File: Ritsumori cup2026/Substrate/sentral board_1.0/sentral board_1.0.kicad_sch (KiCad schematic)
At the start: 9 parts, among them J1 Conn_02x10_Odd_Even, J2 Conn_02x05_Counter_Clockwise, J3 Conn_01x04_Socket, J4 Conn_01x05_Socket, J5 Conn_01x02_Socket, J6 Conn_01x02_Socket, J7 Conn_01x02_Socket, J8 Conn_01x02_Socket, J9 Conn_01x04_Socket

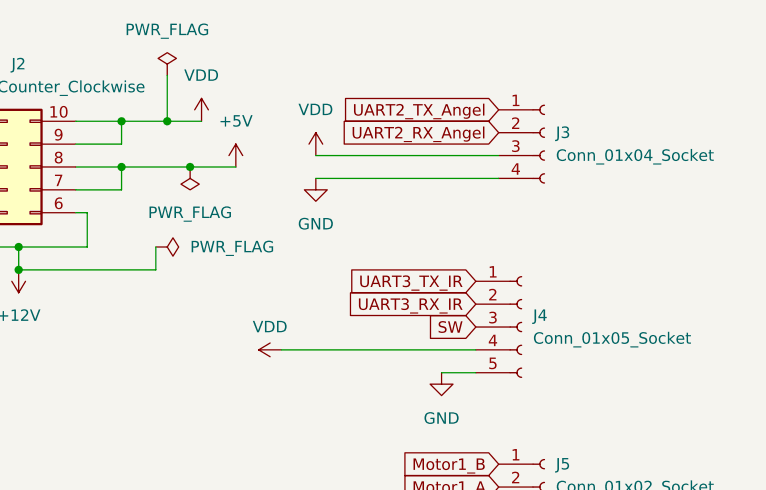
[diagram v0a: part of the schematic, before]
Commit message: Auto Backup: 2026/03/09 13:07:55.49
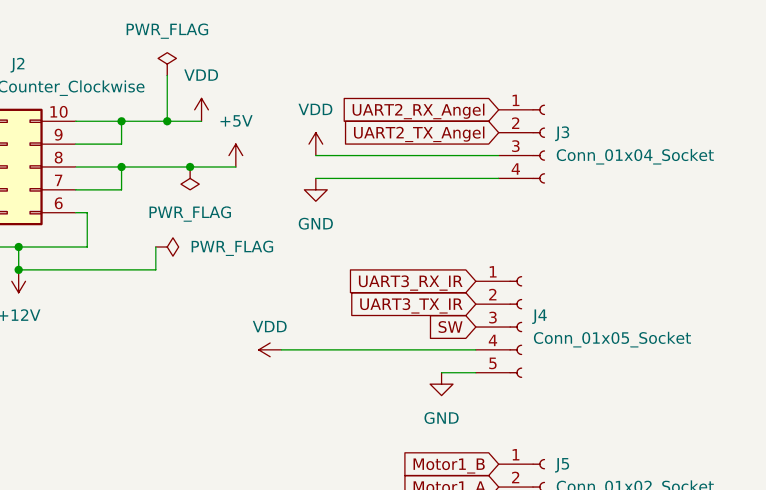
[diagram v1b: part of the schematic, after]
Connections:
- net UART2_RX_Angel: now also J3.1 (Pin_1); no longer J3.2 (Pin_2)
- net UART2_TX_Angel: now also J3.2 (Pin_2); no longer J3.1 (Pin_1)
- net UART3_RX_IR: now also J4.1 (Pin_1); no longer J4.2 (Pin_2)
- net UART3_TX_IR: now also J4.2 (Pin_2); no longer J4.1 (Pin_1)
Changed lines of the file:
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@@
 	(global_label "UART2_RX_Angel"
 		(shape input)
+		(at 228.6 46.99 180)
+		(fields_autoplaced yes)
+		(effects
+			(font
+				(size 1.27 1.27)
+			)
+			(justify right)
+		)
+		(property "Intersheetrefs" "${INTERSHEET_REFS}"
+			(at 210.1935 46.99 0)
+			(effects
+				(font
+					(size 1.27 1.27)
+				)
+				(justify right)
+				(hide yes)
+			)
+		)
+	)
+	(global_label "Motor4_B"
+		(shape input)
+		(at 161.29 85.09 0)
+		(fields_autoplaced yes)
+		(effects
+			(font
+				(size 1.27 1.27)
+			)
+			(justify left)
+		)
+		(property "Intersheetrefs" "${INTERSHEET_REFS}"
+			(at 172.9836 85.09 0)
+			(effects
+				(font
+					(size 1.27 1.27)
+				)
+				(justify left)
+				(hide yes)
+			)
+		)
+	)
+	(global_label "Motor2_B"
+		(shape input)
+		(at 228.6 91.44 180)
+		(fields_autoplaced yes)
+		(effects
+			(font
+				(size 1.27 1.27)
+			)
+			(justify right)
+		)
+		(property "Intersheetrefs" "${INTERSHEET_REFS}"
+			(at 216.9064 91.44 0)
+			(effects
+				(font
+					(size 1.27 1.27)
+				)
+				(justify right)
+				(hide yes)
+			)
+		)
+	)
+	(global_label "UART3_TX_IR"
+		(shape input)
+		(at 226.06 68.58 180)
+		(fields_autoplaced yes)
+		(effects
+			(font
+				(size 1.27 1.27)
+			)
+			(justify right)
+		)
+		(property "Intersheetrefs" "${INTERSHEET_REFS}"
+			(at 211.2215 68.58 0)
+			(effects
+				(font
+					(size 1.27 1.27)
+				)
+				(justify right)
+				(hide yes)
+			)
+		)
+	)
+	(global_label "UART3_RX_IR"
+		(shape input)
+		(at 226.06 66.04 180)
+		(fields_autoplaced yes)
+		(effects
+			(font
+				(size 1.27 1.27)
+			)
+			(justify right)
+		)
+		(property "Intersheetrefs" "${INTERSHEET_REFS}"
+			(at 210.9191 66.04 0)
+			(effects
+				(font
+					(size 1.27 1.27)
+				)
+				(justify right)
+				(hide yes)
+			)
+		)
+	)
+	(global_label "Motor1_B"
+		(shape input)
+		(at 228.6 86.36 180)
+		(fields_autoplaced yes)
+		(effects
+			(font
+				(size 1.27 1.27)
+			)
+			(justify right)
+		)
+		(property "Intersheetrefs" "${INTERSHEET_REFS}"
+			(at 216.9064 86.36 0)
+			(effects
+				(font
+					(size 1.27 1.27)
+				)
+				(justify right)
+				(hide yes)
+			)
+		)
+	)
+	(global_label "SW"
+		(shape input)
+		(at 161.29 82.55 0)
+		(fields_autoplaced yes)
+		(effects
+			(font
+				(size 1.27 1.27)
+			)
+			(justify left)
+		)
+		(property "Intersheetrefs" "${INTERSHEET_REFS}"
+			(at 166.9361 82.55 0)
+			(effects
+				(font
+					(size 1.27 1.27)
+				)
+				(justify left)
+				(hide yes)
+			)
+		)
+	)
+	(global_label "Motor2_A"
+		(shape input)
+		(at 228.6 93.98 180)
+		(fields_autoplaced yes)
+		(effects
+			(font
+				(size 1.27 1.27)
+			)
+			(justify right)
+		)
+		(property "Intersheetrefs" "${INTERSHEET_REFS}"
+			(at 217.0878 93.98 0)
+			(effects
+				(font
+					(size 1.27 1.27)
+				)
+				(justify right)
+				(hide yes)
+			)
+		)
+	)
+	(global_label "Motor1_A"
+		(shape input)
+		(at 161.29 102.87 0)
+		(fields_autoplaced yes)
+		(effects
+			(font
+				(size 1.27 1.27)
+			)
+			(justify left)
+		)
+		(property "Intersheetrefs" "${INTERSHEET_REFS}"
+			(at 172.8022 102.87 0)
+			(effects
+				(font
+					(size 1.27 1.27)
+				)
+				(justify left)
+				(hide yes)
+			)
+		)
+	)
+	(global_label "Motor3_B"
+		(shape input)
+		(at 228.6 96.52 180)
+		(fields_autoplaced yes)
+		(effects
+			(font
+				(size 1.27 1.27)
+			)
+			(justify right)
+		)
+		(property "Intersheetrefs" "${INTERSHEET_REFS}"
+			(at 216.9064 96.52 0)
+			(effects
+				(font
+					(size 1.27 1.27)
+				)
+				(justify right)
+				(hide yes)
+			)
+		)
+	)
+	(global_label "UART2_TX_Angel"
+		(shape input)
 		(at 228.6 49.53 180)
 		(fields_autoplaced yes)
@@
 		)
 		(property "Intersheetrefs" "${INTERSHEET_REFS}"
-			(at 210.1935 49.53 0)
-			(effects
-				(font
-					(size 1.27 1.27)
-				)
-				(justify right)
-				(hide yes)
-			)
-		)
-	)
-	(global_label "Motor4_B"
-		(shape input)
-		(at 161.29 85.09 0)
-		(fields_autoplaced yes)
-		(effects
-			(font
-				(size 1.27 1.27)
-			)
-			(justify left)
-		)
-		(property "Intersheetrefs" "${INTERSHEET_REFS}"
-			(at 172.9836 85.09 0)
-			(effects
-				(font
-					(size 1.27 1.27)
-				)
-				(justify left)
-				(hide yes)
-			)
-		)
-	)
-	(global_label "Motor2_B"
-		(shape input)
-		(at 228.6 91.44 180)
-		(fields_autoplaced yes)
-		(effects
-			(font
-				(size 1.27 1.27)
-			)
-			(justify right)
-		)
-		(property "Intersheetrefs" "${INTERSHEET_REFS}"
-			(at 216.9064 91.44 0)
-			(effects
-				(font
-					(size 1.27 1.27)
-				)
-				(justify right)
-				(hide yes)
-			)
-		)
-	)
-	(global_label "UART3_TX_IR"
-		(shape input)
-		(at 226.06 66.04 180)
-		(fields_autoplaced yes)
-		(effects
-			(font
-				(size 1.27 1.27)
-			)
-			(justify right)
-		)
-		(property "Intersheetrefs" "${INTERSHEET_REFS}"
-			(at 211.2215 66.04 0)
-			(effects
-				(font
-					(size 1.27 1.27)
-				)
-				(justify right)
-				(hide yes)
-			)
-		)
-	)
-	(global_label "UART3_RX_IR"
-		(shape input)
-		(at 226.06 68.58 180)
-		(fields_autoplaced yes)
-		(effects
-			(font
-				(size 1.27 1.27)
-			)
-			(justify right)
-		)
-		(property "Intersheetrefs" "${INTERSHEET_REFS}"
-			(at 210.9191 68.58 0)
-			(effects
-				(font
-					(size 1.27 1.27)
-				)
-				(justify right)
-				(hide yes)
-			)
-		)
-	)
-	(global_label "Motor1_B"
-		(shape input)
-		(at 228.6 86.36 180)
-		(fields_autoplaced yes)
-		(effects
-			(font
-				(size 1.27 1.27)
-			)
-			(justify right)
-		)
-		(property "Intersheetrefs" "${INTERSHEET_REFS}"
-			(at 216.9064 86.36 0)
-			(effects
-				(font
-					(size 1.27 1.27)
-				)
-				(justify right)
-				(hide yes)
-			)
-		)
-	)
-	(global_label "SW"
-		(shape input)
-		(at 161.29 82.55 0)
-		(fields_autoplaced yes)
-		(effects
-			(font
-				(size 1.27 1.27)
-			)
-			(justify left)
-		)
-		(property "Intersheetrefs" "${INTERSHEET_REFS}"
-			(at 166.9361 82.55 0)
-			(effects
-				(font
-					(size 1.27 1.27)
-				)
-				(justify left)
-				(hide yes)
-			)
-		)
-	)
-	(global_label "Motor2_A"
-		(shape input)
-		(at 228.6 93.98 180)
-		(fields_autoplaced yes)
-		(effects
-			(font
-				(size 1.27 1.27)
-			)
-			(justify right)
-		)
-		(property "Intersheetrefs" "${INTERSHEET_REFS}"
-			(at 217.0878 93.98 0)
-			(effects
-				(font
-					(size 1.27 1.27)
-				)
-				(justify right)
-				(hide yes)
-			)
-		)
-	)
-	(global_label "Motor1_A"
-		(shape input)
-		(at 161.29 102.87 0)
-		(fields_autoplaced yes)
-		(effects
-			(font
-				(size 1.27 1.27)
-			)
-			(justify left)
-		)
-		(property "Intersheetrefs" "${INTERSHEET_REFS}"
-			(at 172.8022 102.87 0)
-			(effects
-				(font
-					(size 1.27 1.27)
-				)
-				(justify left)
-				(hide yes)
-			)
-		)
-	)
-	(global_label "Motor3_B"
-		(shape input)
-		(at 228.6 96.52 180)
-		(fields_autoplaced yes)
-		(effects
-			(font
-				(size 1.27 1.27)
-			)
-			(justify right)
-		)
-		(property "Intersheetrefs" "${INTERSHEET_REFS}"
-			(at 216.9064 96.52 0)
-			(effects
-				(font
-					(size 1.27 1.27)
-				)
-				(justify right)
-				(hide yes)
-			)
-		)
-	)
-	(global_label "UART2_TX_Angel"
-		(shape input)
-		(at 228.6 46.99 180)
-		(fields_autoplaced yes)
-		(effects
-			(font
-				(size 1.27 1.27)
-			)
-			(justify right)
-		)
-		(property "Intersheetrefs" "${INTERSHEET_REFS}"
-			(at 210.4959 46.99 0)
-			(effects
-				(font
+			(at 210.4959 49.53 0)
+			(effects
+				(font
